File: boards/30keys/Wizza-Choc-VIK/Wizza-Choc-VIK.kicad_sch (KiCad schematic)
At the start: 80 parts, among them J1 AudioJack4dpb, J11 Conn_01x05, J2 AudioJack4dpb, J3 Conn_01x03_Socket, J4 Conn_01x03_Socket, J9 Conn_01x05, SW1 SW_Push, SW10 SW_Push, SW11 SW_Push, SW12 SW_Push, SW13 SW_Push, SW14 SW_Push, SW15 SW_Push, SW16 SW_Push, SW17 SW_Push, SW18 SW_Push, SW19 SW_Push, SW2 SW_Push, SW20 SW_Push, SW21 SW_Push, SW22 SW_Push, SW23 SW_Push, SW24 SW_Push, SW25 SW_SPDT, SW26 SW_Push, SW27 SW_Push, SW28 SW_Push, SW29 SW_Push, SW3 SW_Push, SW30 SW_SPDT, SW31 SW_Push, SW32 SW_Push, SW33 SW_Push, SW34 Rotary_Encoder_Switch, SW35 Rotary_Encoder_Switch, SW4 SW_Push, SW40 SW_Push, SW5 SW_Push, SW6 SW_Push, SW7 SW_Push, SW8 SW_Push, SW9 SW_Push, U3 Helios, U4 Helios

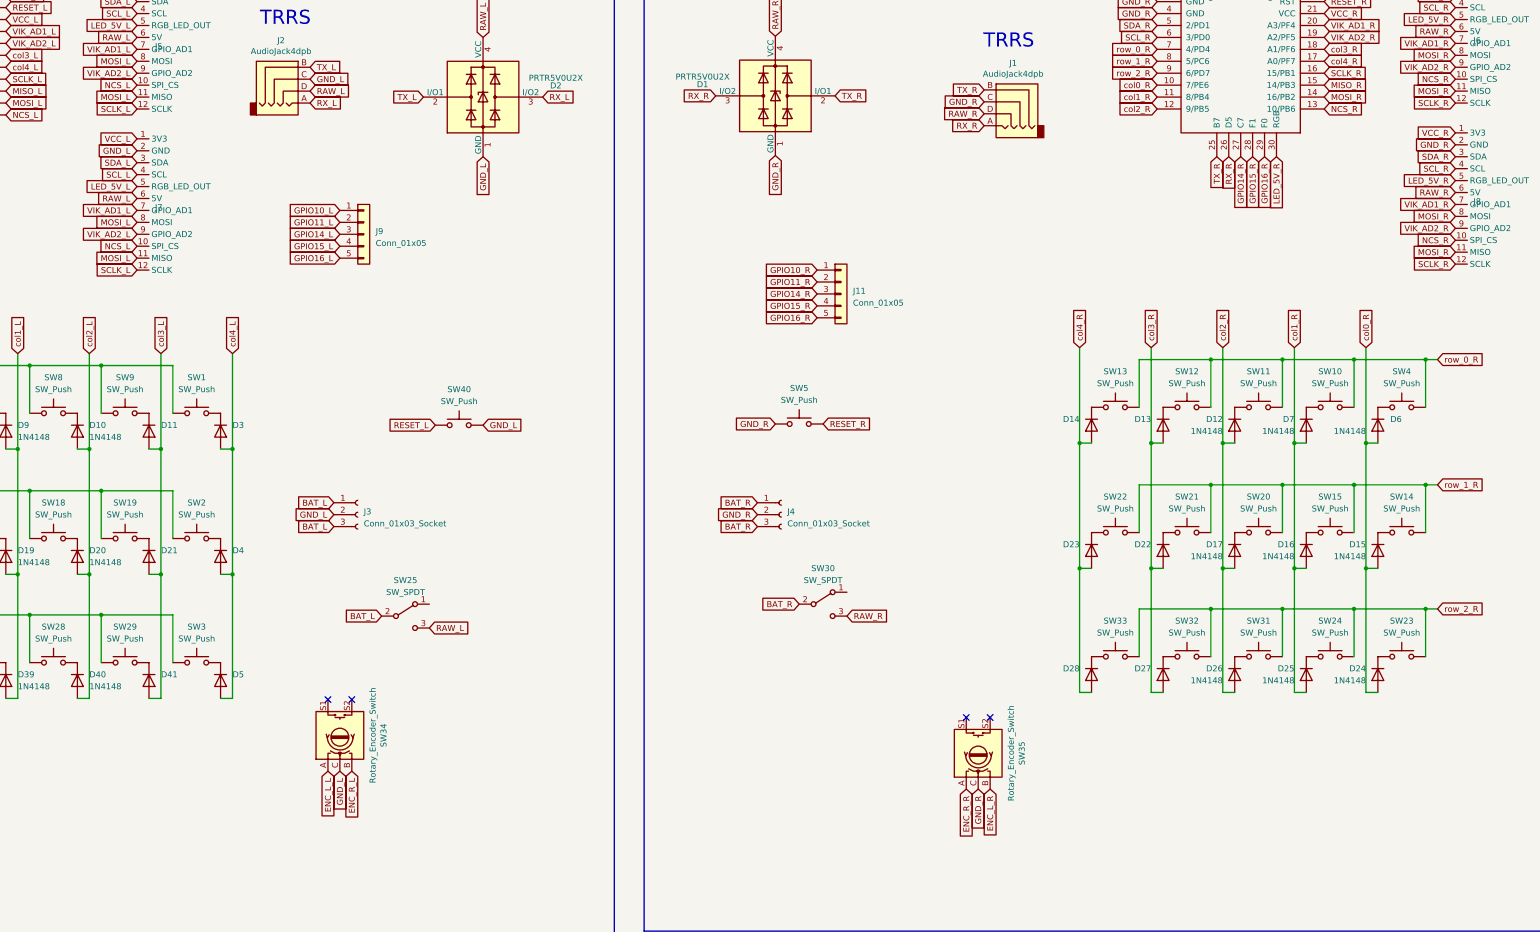
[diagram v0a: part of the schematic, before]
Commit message: wizza vik
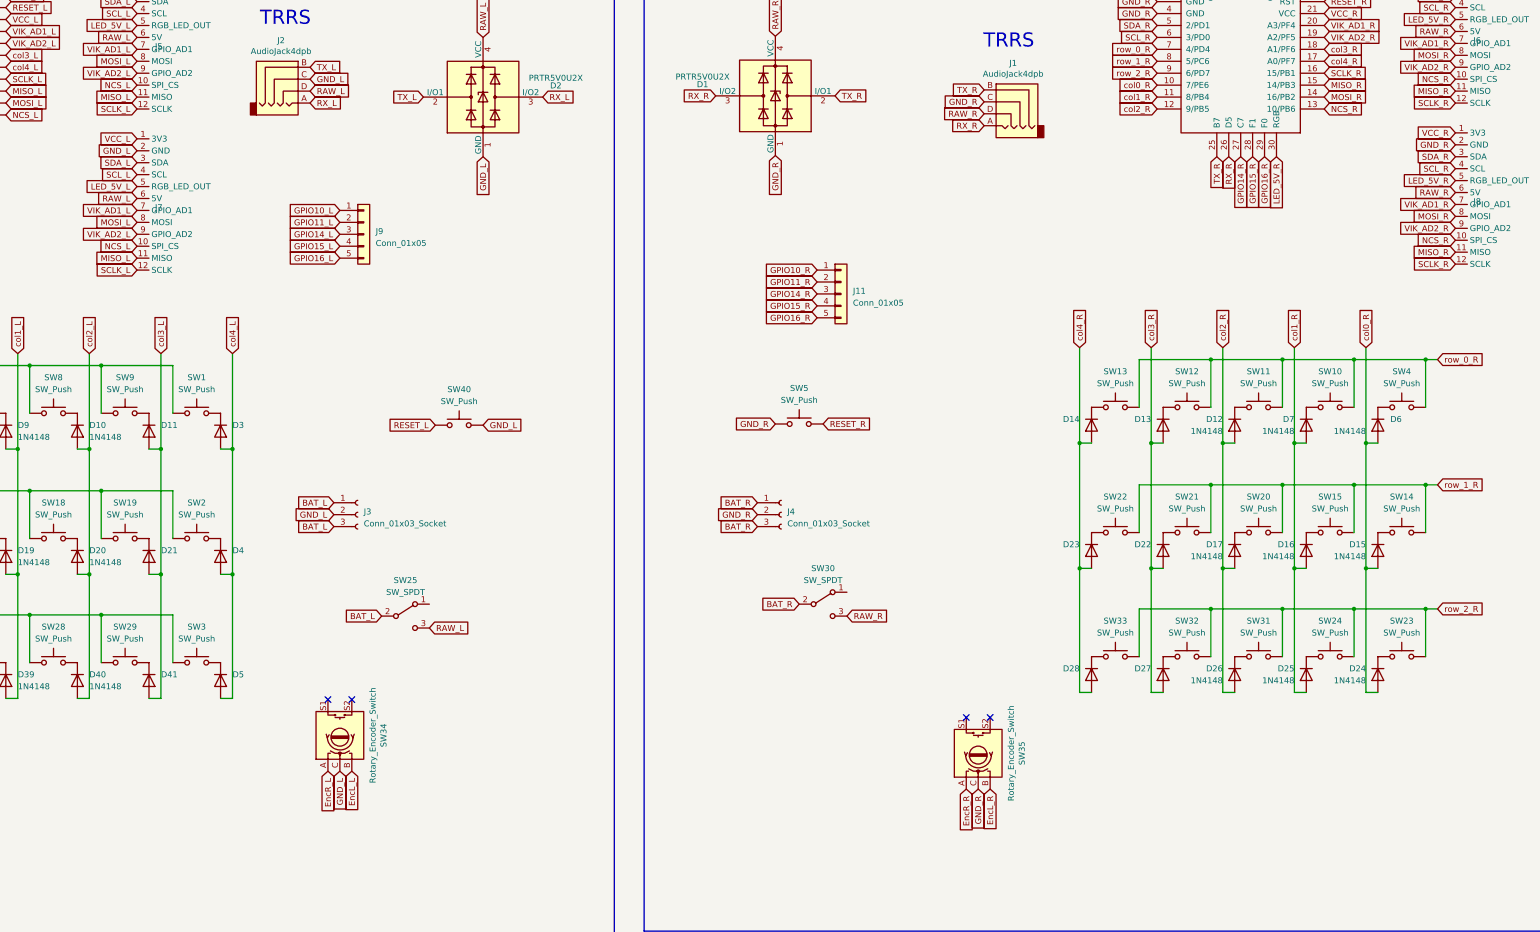
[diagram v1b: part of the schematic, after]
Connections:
- net ENC_L_L is gone; now on net EncR_L: SW34.A
- net ENC_L_R is gone; now on net EncL_R: SW35.B
- net ENC_R_L is gone; now on net EncL_L: SW34.B
- net ENC_R_R is gone; now on net EncR_R: SW35.A
- net MISO_L: now also J5.11 (MISO), J7.11 (MISO)
- net MISO_R: now also J6.11 (MISO), J8.11 (MISO)
- net MOSI_L: no longer J5.11 (MISO), J7.11 (MISO)
- net MOSI_R: no longer J6.11 (MISO), J8.11 (MISO)
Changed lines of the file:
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@@
+    )
+  )
+  (global_label "EncL_L" (shape input) (at 151.13 229.87 270) (fields_autoplaced)
+    (effects (font (size 1.27 1.27)) (justify right))
+    (property "Intersheetrefs" "${INTERSHEET_REFS}" (at 151.13 239.1862 90)
+      (effects (font (size 1.27 1.27)) (justify right) hide)
     )
   )
@@
     )
   )
+  (global_label "EncL_R" (shape input) (at 287.02 233.68 270) (fields_autoplaced)
+    (effects (font (size 1.27 1.27)) (justify right))
+    (property "Intersheetrefs" "${INTERSHEET_REFS}" (at 287.02 243.2381 90)
+      (effects (font (size 1.27 1.27)) (justify right) hide)
+    )
+  )
   (global_label "SDA_L" (shape input) (at 105.41 66.04 180) (fields_autoplaced)
     (effects (font (size 1.27 1.27)) (justify right))
@@
     )
   )
+  (global_label "MISO_R" (shape input) (at 386.08 119.38 180) (fields_autoplaced)
+    (effects (font (size 1.27 1.27)) (justify right))
+    (property "Intersheetrefs" "${INTERSHEET_REFS}" (at 376.3404 119.38 0)
+      (effects (font (size 1.27 1.27)) (justify right) hide)
+    )
+  )
   (global_label "col1_R" (shape input) (at 351.79 139.7 90) (fields_autoplaced)
     (effects (font (size 1.27 1.27)) (justify left))
@@
     (effects (font (size 1.27 1.27)) (justify right))
     (property "Intersheetrefs" "${INTERSHEET_REFS}" (at 93.0094 110.49 0)
+      (effects (font (size 1.27 1.27)) (justify right) hide)
+    )
+  )
+  (global_label "MISO_R" (shape input) (at 386.08 85.09 180) (fields_autoplaced)
+    (effects (font (size 1.27 1.27)) (justify right))
+    (property "Intersheetrefs" "${INTERSHEET_REFS}" (at 376.3404 85.09 0)
       (effects (font (size 1.27 1.27)) (justify right) hide)
     )
@@
     )
   )
-  (global_label "ENC_L_L" (shape input) (at 146.05 229.87 270) (fields_autoplaced)
-    (effects (font (size 1.27 1.27)) (justify right))
-    (property "Intersheetrefs" "${INTERSHEET_REFS}" (at 146.05 240.5167 90)
-      (effects (font (size 1.27 1.27)) (justify right) hide)
-    )
-  )
   (global_label "row_1_R" (shape input) (at 382.27 168.91 0) (fields_autoplaced)
     (effects (font (size 1.27 1.27)) (justify left))
@@
     (effects (font (size 1.27 1.27)) (justify right))
     (property "Intersheetrefs" "${INTERSHEET_REFS}" (at 347.98 110.9162 90)
-      (effects (font (size 1.27 1.27)) (justify right) hide)
-    )
-  )
-  (global_label "MOSI_R" (shape input) (at 386.08 85.09 180) (fields_autoplaced)
-    (effects (font (size 1.27 1.27)) (justify right))
-    (property "Intersheetrefs" "${INTERSHEET_REFS}" (at 376.3404 85.09 0)
       (effects (font (size 1.27 1.27)) (justify right) hide)
     )
@@
     )
   )
-  (global_label "ENC_L_R" (shape input) (at 287.02 233.68 270) (fields_autoplaced)
-    (effects (font (size 1.27 1.27)) (justify right))
-    (property "Intersheetrefs" "${INTERSHEET_REFS}" (at 287.02 244.5686 90)
-      (effects (font (size 1.27 1.27)) (justify right) hide)
-    )
-  )
   (global_label "GND_L" (shape input) (at 179.07 156.21 0) (fields_autoplaced)
     (effects (font (size 1.27 1.27)) (justify left))
@@
     )
   )
-  (global_label "MOSI_L" (shape input) (at 105.41 120.65 180) (fields_autoplaced)
-    (effects (font (size 1.27 1.27)) (justify right))
-    (property "Intersheetrefs" "${INTERSHEET_REFS}" (at 95.9123 120.65 0)
-      (effects (font (size 1.27 1.27)) (justify right) hide)
-    )
-  )
   (global_label "RAW_L" (shape input) (at 142.24 85.09 0)
     (effects (font (size 1.27 1.27)) (justify left))
@@
     )
   )
-  (global_label "MOSI_R" (shape input) (at 386.08 119.38 180) (fields_autoplaced)
-    (effects (font (size 1.27 1.27)) (justify right))
-    (property "Intersheetrefs" "${INTERSHEET_REFS}" (at 376.3404 119.38 0)
-      (effects (font (size 1.27 1.27)) (justify right) hide)
-    )
-  )
   (global_label "RAW_L" (shape input) (at 167.64 199.39 0) (fields_autoplaced)
     (effects (font (size 1.27 1.27)) (justify left))
@@
     )
   )
-  (global_label "ENC_R_R" (shape input) (at 281.94 233.68 270) (fields_autoplaced)
-    (effects (font (size 1.27 1.27)) (justify right))
-    (property "Intersheetrefs" "${INTERSHEET_REFS}" (at 281.94 244.8105 90)
-      (effects (font (size 1.27 1.27)) (justify right) hide)
-    )
-  )
   (global_label "LED_5V_R" (shape input) (at 386.08 104.14 180) (fields_autoplaced)
     (effects (font (size 1.27 1.27)) (justify right))
@@
     )
   )
+  (global_label "MISO_L" (shape input) (at 105.41 120.65 180) (fields_autoplaced)
+    (effects (font (size 1.27 1.27)) (justify right))
+    (property "Intersheetrefs" "${INTERSHEET_REFS}" (at 95.9123 120.65 0)
+      (effects (font (size 1.27 1.27)) (justify right) hide)
+    )
+  )
   (global_label "VIK_AD1_L" (shape input) (at 77.47 72.39 0) (fields_autoplaced)
     (effects (font (size 1.27 1.27)) (justify left))
@@
     )
   )
+  (global_label "EncR_R" (shape input) (at 281.94 233.68 270) (fields_autoplaced)
+    (effects (font (size 1.27 1.27)) (justify right))
+    (property "Intersheetrefs" "${INTERSHEET_REFS}" (at 281.94 243.48 90)
+      (effects (font (size 1.27 1.27)) (justify right) hide)
+    )
+  )
   (global_label "VCC_R" (shape input) (at 386.08 93.98 180) (fields_autoplaced)
     (effects (font (size 1.27 1.27)) (justify right))
@@
     (property "Intersheetrefs" "${INTERSHEET_REFS}" (at 367.1539 63.5 0)
       (effects (font (size 1.27 1.27)) (justify left) hide)
-    )
-  )
-  (global_label "ENC_R_L" (shape input) (at 151.13 229.87 270) (fields_autoplaced)
-    (effects (font (size 1.27 1.27)) (justify right))
-    (property "Intersheetrefs" "${INTERSHEET_REFS}" (at 151.13 240.7586 90)
-      (effects (font (size 1.27 1.27)) (justify right) hide)
     )
   )
@@
     )
   )
+  (global_label "MISO_L" (shape input) (at 105.41 86.36 180) (fields_autoplaced)
+    (effects (font (size 1.27 1.27)) (justify right))
+    (property "Intersheetrefs" "${INTERSHEET_REFS}" (at 95.9123 86.36 0)
+      (effects (font (size 1.27 1.27)) (justify right) hide)
+    )
+  )
   (global_label "TX_L" (shape input) (at 142.24 80.01 0) (fields_autoplaced)
     (effects (font (size 1.27 1.27)) (justify left))
@@
     )
   )
+  (global_label "EncR_L" (shape input) (at 146.05 229.87 270) (fields_autoplaced)
+    (effects (font (size 1.27 1.27)) (justify right))
+    (property "Intersheetrefs" "${INTERSHEET_REFS}" (at 146.05 239.4281 90)
+      (effects (font (size 1.27 1.27)) (justify right) hide)
+    )
+  )
   (global_label "RX_R" (shape input) (at 285.75 92.456 180) (fields_autoplaced)
     (effects (font (size 1.27 1.27)) (justify right))
@@
       (effects (font (size 1.27 1.27)) (justify right) hide)
     )
-  )
-  (global_label "MOSI_L" (shape input) (at 105.41 86.36 180) (fields_autoplaced)
-    (effects (font (size 1.27 1.27)) (justify right))
-    (property "Intersheetrefs" "${INTERSHEET_REFS}" (at 95.9123 86.36 0)
-      (effects (font (size 1.27 1.27)) (justify right) hide)
-    )
